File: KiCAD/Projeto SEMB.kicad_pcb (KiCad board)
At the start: 2 copper layers, 114 x 39 mm, 64 parts, among them J1 Battery-12V, J2 ST-Link V2, M1 Motor_DC, Q2 IRLML5203, SW1 Reset, SW2 BOOT_0, SW3 SW_SPDT, SW4 User Button, U1 STM32F411CEUx, U10 XL4015, U11 LCD-016N002L, U13 INA333xxDGK, U2 2SMPP-03, U3 TLV2371P, U4 DRV8212P, U5 PCF8574A, U7 TPS7A2433DBVR, Y1 LSE

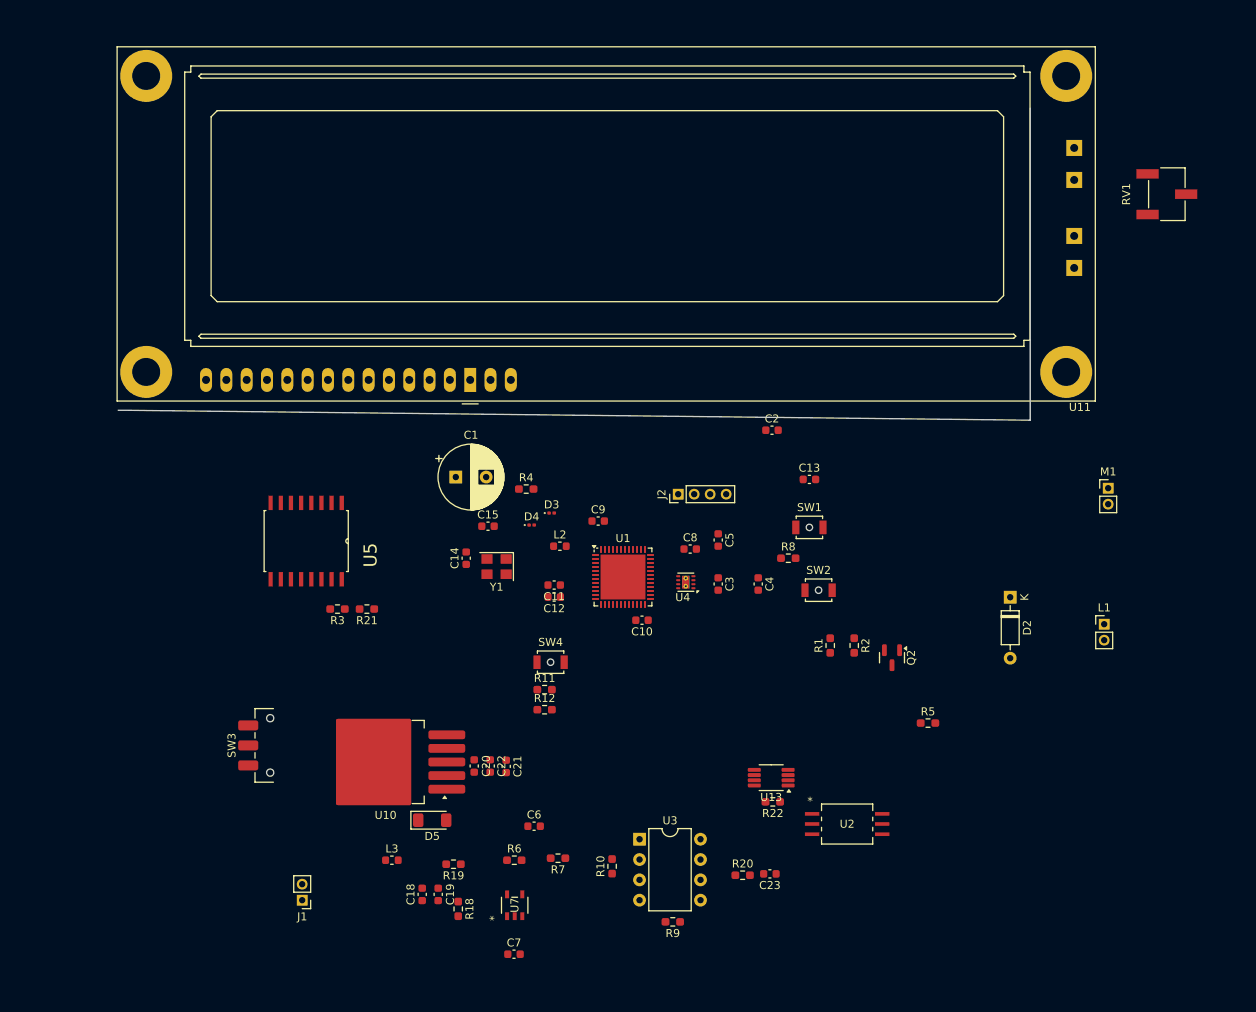
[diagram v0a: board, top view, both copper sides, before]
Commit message: User Interface
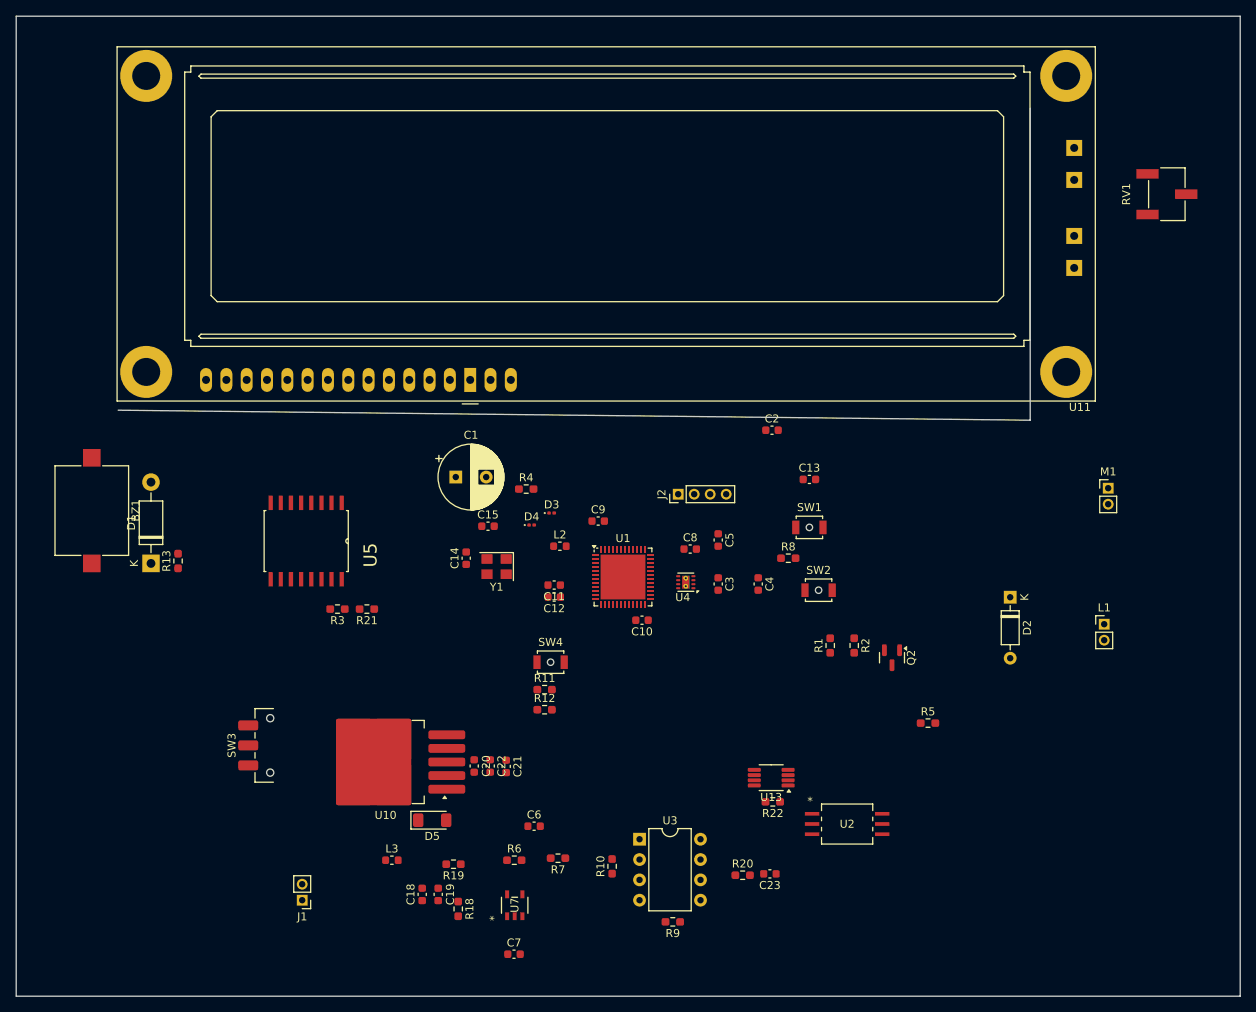
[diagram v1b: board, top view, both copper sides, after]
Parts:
- added BZ1: Buzzer, Buzzer_Beeper:Buzzer_Mallory_AST1109MLTRQ, F.Cu at (84.2, 77.0)
- added D1: 1N4007, Diode_THT:D_DO-41_SOD81_P10.16mm_Horizontal, F.Cu at (91.6, 83.7)
- added R13: 100R, Resistor_SMD:R_0603_1608Metric_Pad0.98x0.95mm_HandSolder, F.Cu at (95.0, 83.3)
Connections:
- U1 pad 31: unconnected-(U1-PA10-Pad31) -> PA10
- U1 pad 5: PH0 -> unconnected-(U1-PH0-Pad5)
- U1 pad 6: PH1 -> unconnected-(U1-PH1-Pad6)
- U5 pad 13: unconnected-(U5-~{INT}-Pad13) -> +5V
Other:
- board size 114 x 39 mm -> 153 x 122.5 mm
